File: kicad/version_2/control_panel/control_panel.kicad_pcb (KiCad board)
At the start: 2 copper layers, 111 x 69 mm, 41 parts, among them J1 Conn_01x01_Pin, J2 Conn_01x01_Pin, J3 Conn_01x01_Pin, J4 Conn_01x01_Pin, SW1 SW_Push

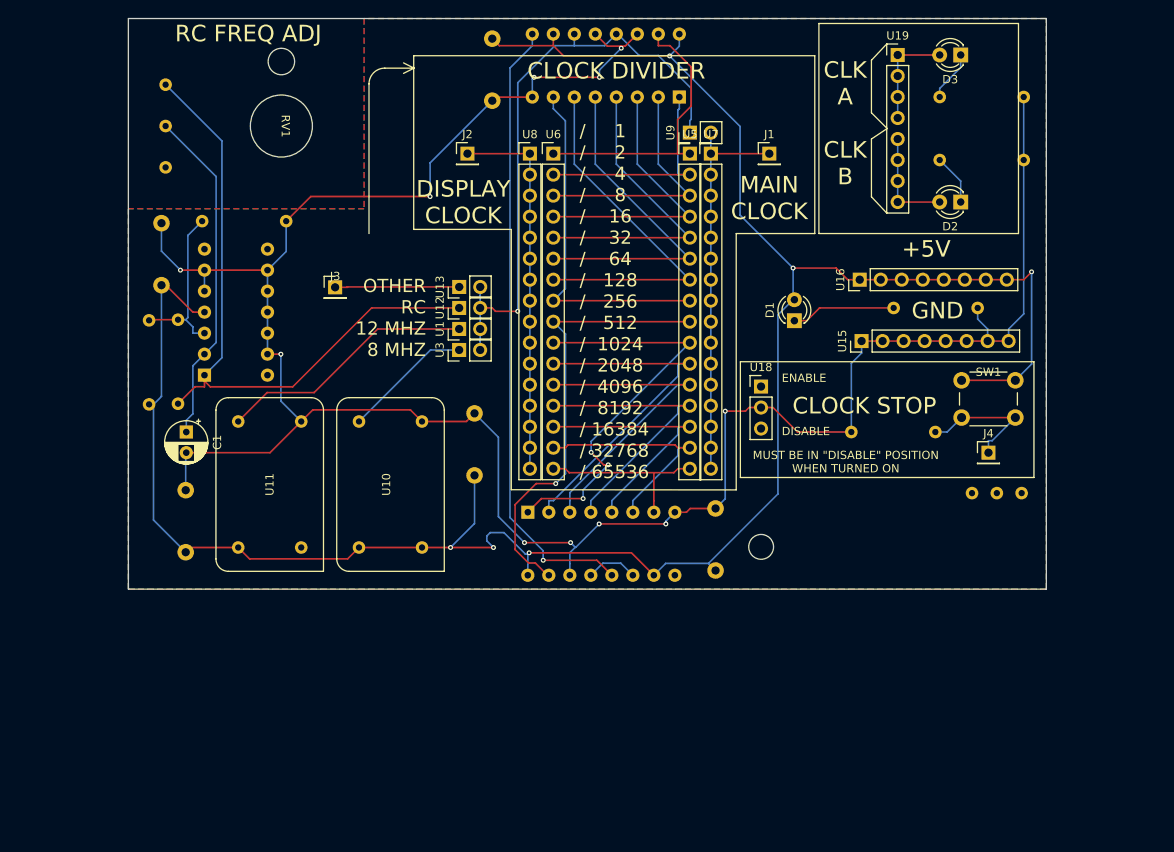
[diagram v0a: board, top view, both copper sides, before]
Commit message: Finished control panel
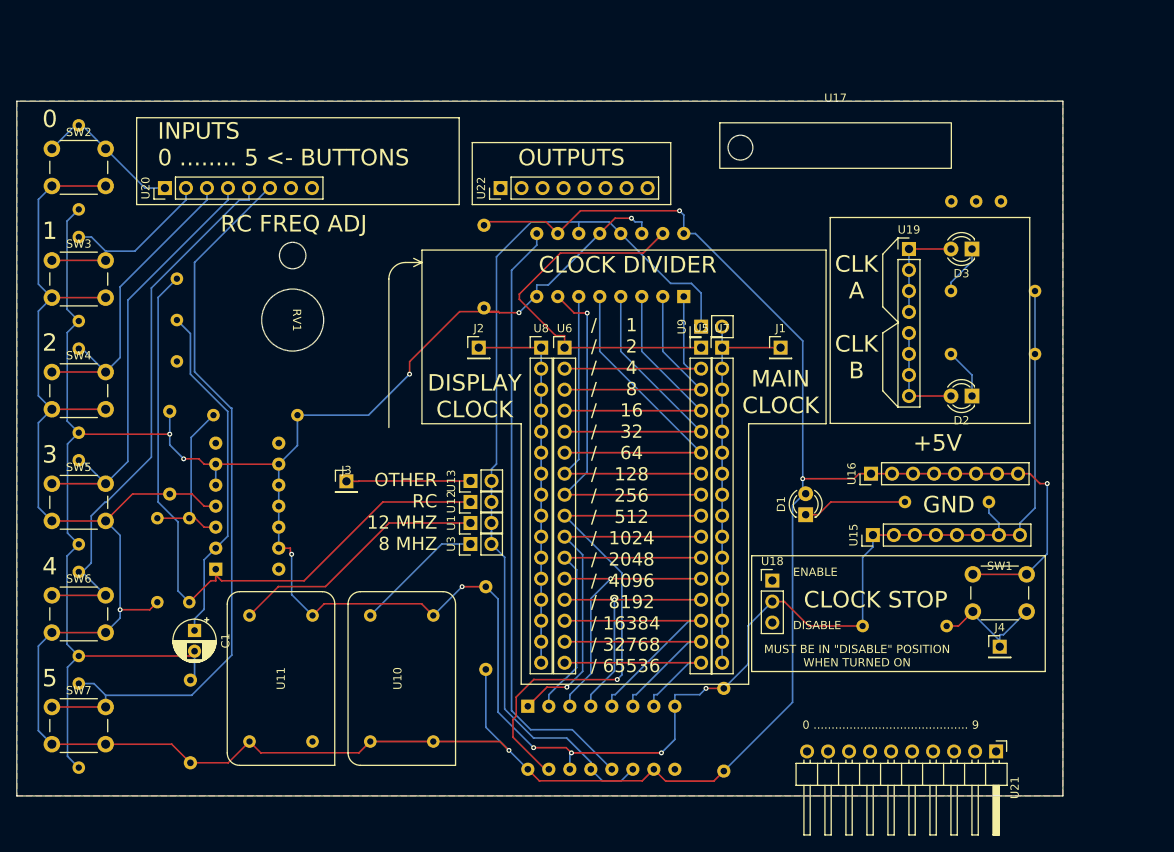
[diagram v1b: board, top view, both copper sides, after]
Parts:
- added R10: R, custom_footprint_library:0.4_pitch_resistor, B.Cu at (62.0, 82.0)
- added R11: R, custom_footprint_library:0.4_pitch_resistor, B.Cu at (62.0, 95.5)
- added R12: R, custom_footprint_library:0.4_pitch_resistor, B.Cu at (62.0, 109.0)
- added R13: R, custom_footprint_library:0.4_pitch_resistor, B.Cu at (62.0, 122.5)
- added R8: R, custom_footprint_library:0.4_pitch_resistor, B.Cu at (62.0, 55.0)
- added R9: R, custom_footprint_library:0.4_pitch_resistor, B.Cu at (62.0, 68.5)
- added SW2: SW_Push, Button_Switch_THT:SW_PUSH_6mm, F.Cu at (58.8, 52.8)
- added SW3: SW_Push, Button_Switch_THT:SW_PUSH_6mm, F.Cu at (58.8, 66.2)
- added SW4: SW_Push, Button_Switch_THT:SW_PUSH_6mm, F.Cu at (58.8, 79.8)
- added SW5: SW_Push, Button_Switch_THT:SW_PUSH_6mm, F.Cu at (58.8, 93.2)
- added SW6: SW_Push, Button_Switch_THT:SW_PUSH_6mm, F.Cu at (58.8, 106.8)
- added SW7: SW_Push, Button_Switch_THT:SW_PUSH_6mm, F.Cu at (58.8, 120.2)
- added U20: ~, Connector_PinHeader_2.54mm:PinHeader_1x08_P2.54mm_Vertical, F.Cu at (72.4, 57.5)
- added U21: ~, Connector_PinHeader_2.54mm:PinHeader_1x10_P2.54mm_Horizontal, F.Cu at (172.9, 125.6)
- added U22: ~, Connector_PinHeader_2.54mm:PinHeader_1x08_P2.54mm_Vertical, F.Cu at (113.0, 57.5)
- C2, C3, C4, C5, C6: footprint Capacitor_THT:C_Rect_L10.3mm_W4.5mm_P7.50mm_MKS4 -> Capacitor_THT:C_Rect_L11.0mm_W4.2mm_P10.00mm_MKT
- U17: moved to F.Cu
- moved U17 59.3 mm to (153.5, 47.1)
- moved C3 25.5 mm to (75.5, 127.0)
- moved C6 25.3 mm to (73.0, 94.5)
- moved C5 24.3 mm to (140.0, 128.0)
- moved U2 24.1 mm to (135.2, 70.6)
- moved R5 24.0 mm to (75.4, 102.5)
- moved C1 24.0 mm to (76.0, 111.0)
- moved R3 23.9 mm to (71.5, 102.5)
- moved U10 23.5 mm to (101.1, 116.8)
- moved U13 23.5 mm to (109.4, 92.9)
- moved U16 23.5 mm to (157.8, 92.0)
- moved U9 23.5 mm to (137.3, 74.3)
- moved D2 23.5 mm to (170.0, 82.7)
- moved D3 23.5 mm to (170.0, 64.9)
- moved R7 23.5 mm to (172.6, 70.0)
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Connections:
- U4 pad 11: Net-(U4-CCLK) -> Net-(U1-B)
- U4 pad 13: Net-(U4-CCLK) -> Net-(U1-B)
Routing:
- net Net-(D1-A): track 274.3 -> 379.4 mm, vias 6 -> 5
- net Net-(U20-5): track 0.00 -> 91.3 mm
- net Net-(U10-GND): track 290.2 -> 373.9 mm
- net Net-(U20-4): track 0.00 -> 66.5 mm
- net Net-(U20-3): track 0.00 -> 52.8 mm
- net Net-(U1-B): track 72.9 -> 111.3 mm, vias 1 -> 0
- net Net-(U20-2): track 0.00 -> 38.2 mm
- net Net-(U20-1): track 0.00 -> 25.3 mm
- net Net-(U20-0): track 0.00 -> 18.0 mm
- net Net-(U2-Q0): track 34.1 -> 46.3 mm
- net Net-(U4-Q0): track 54.0 -> 63.5 mm
- net Net-(U4-Q1): track 50.1 -> 42.1 mm, vias 3 -> 1
- net Net-(U4-CCLK): track 6.29 -> 0.00 mm
- net Net-(U4-Q2): track 42.7 -> 36.5 mm
- net Net-(U2-Q6): track 44.4 -> 38.6 mm
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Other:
- board size 111 x 69 mm -> 126.5 x 84 mm
- board text added: "0 ........................................... 9"
- board text added: "0 1 2 3 4 5"
- board text added: "INPUTS 0 ........ 5 <- BUTTONS"
- board text added: "OUTPUTS"
